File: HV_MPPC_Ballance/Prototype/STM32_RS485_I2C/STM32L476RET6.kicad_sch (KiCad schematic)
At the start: 10 parts, among them SW1 SW_Push, U1 STM32L476RET6

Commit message: .
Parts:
- C1, C2, C3, C4, C5, C6: footprint Capacitor_SMD:C_0402_1005Metric -> 0_lib:0402_density_C_Capacitor
- R1, R2: footprint Resistor_SMD:R_0402_1005Metric -> 0_lib:0402_density_C_Resistor
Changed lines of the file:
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@@
 			)
 		)
-		(property "Footprint" "Resistor_SMD:R_0402_1005Metric"
+		(property "Footprint" "0_lib:0402_density_C_Resistor"
 			(at 37.592 55.88 90)
 			(effects
@@
 			)
 		)
-		(property "Footprint" "Capacitor_SMD:C_0402_1005Metric"
+		(property "Footprint" "0_lib:0402_density_C_Capacitor"
 			(at 70.8152 31.75 0)
 			(effects
@@
 			)
 		)
-		(property "Footprint" "Capacitor_SMD:C_0402_1005Metric"
+		(property "Footprint" "0_lib:0402_density_C_Capacitor"
 			(at 83.5152 31.75 0)
 			(effects
@@
 			)
 		)
-		(property "Footprint" "Capacitor_SMD:C_0402_1005Metric"
+		(property "Footprint" "0_lib:0402_density_C_Capacitor"
 			(at 58.1152 31.75 0)
 			(effects
@@
 			)
 		)
-		(property "Footprint" "Capacitor_SMD:C_0402_1005Metric"
+		(property "Footprint" "0_lib:0402_density_C_Capacitor"
 			(at 89.8652 31.75 0)
 			(effects
@@
 			)
 		)
-		(property "Footprint" "Capacitor_SMD:C_0402_1005Metric"
+		(property "Footprint" "0_lib:0402_density_C_Capacitor"
 			(at 77.1652 31.75 0)
 			(effects
@@
 			)
 		)
-		(property "Footprint" "Capacitor_SMD:C_0402_1005Metric"
+		(property "Footprint" "0_lib:0402_density_C_Capacitor"
 			(at 64.4652 31.75 0)
 			(effects
@@
 			)
 		)
-		(property "Footprint" "Resistor_SMD:R_0402_1005Metric"
+		(property "Footprint" "0_lib:0402_density_C_Resistor"
 			(at 43.942 69.85 90)
 			(effects

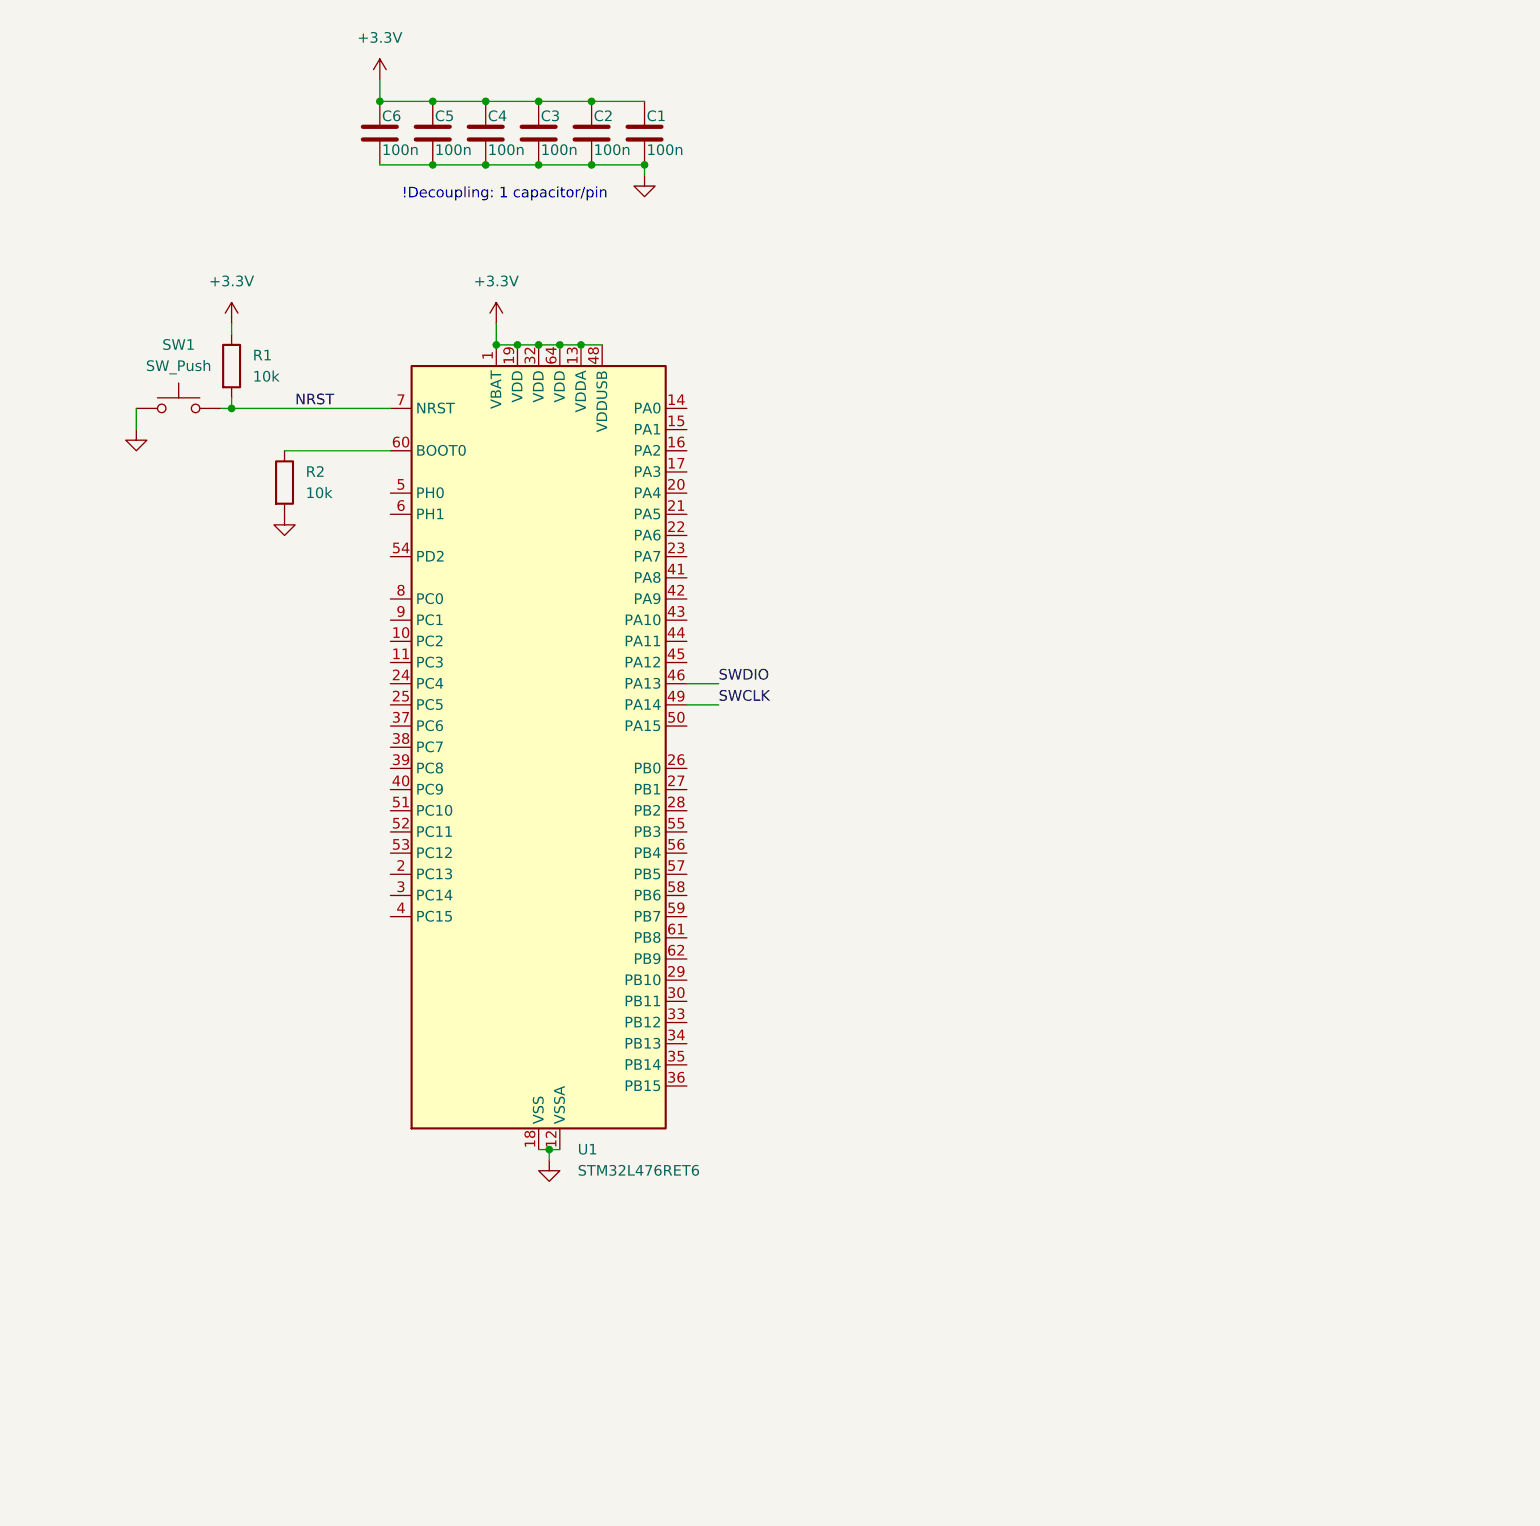
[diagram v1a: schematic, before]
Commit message: .
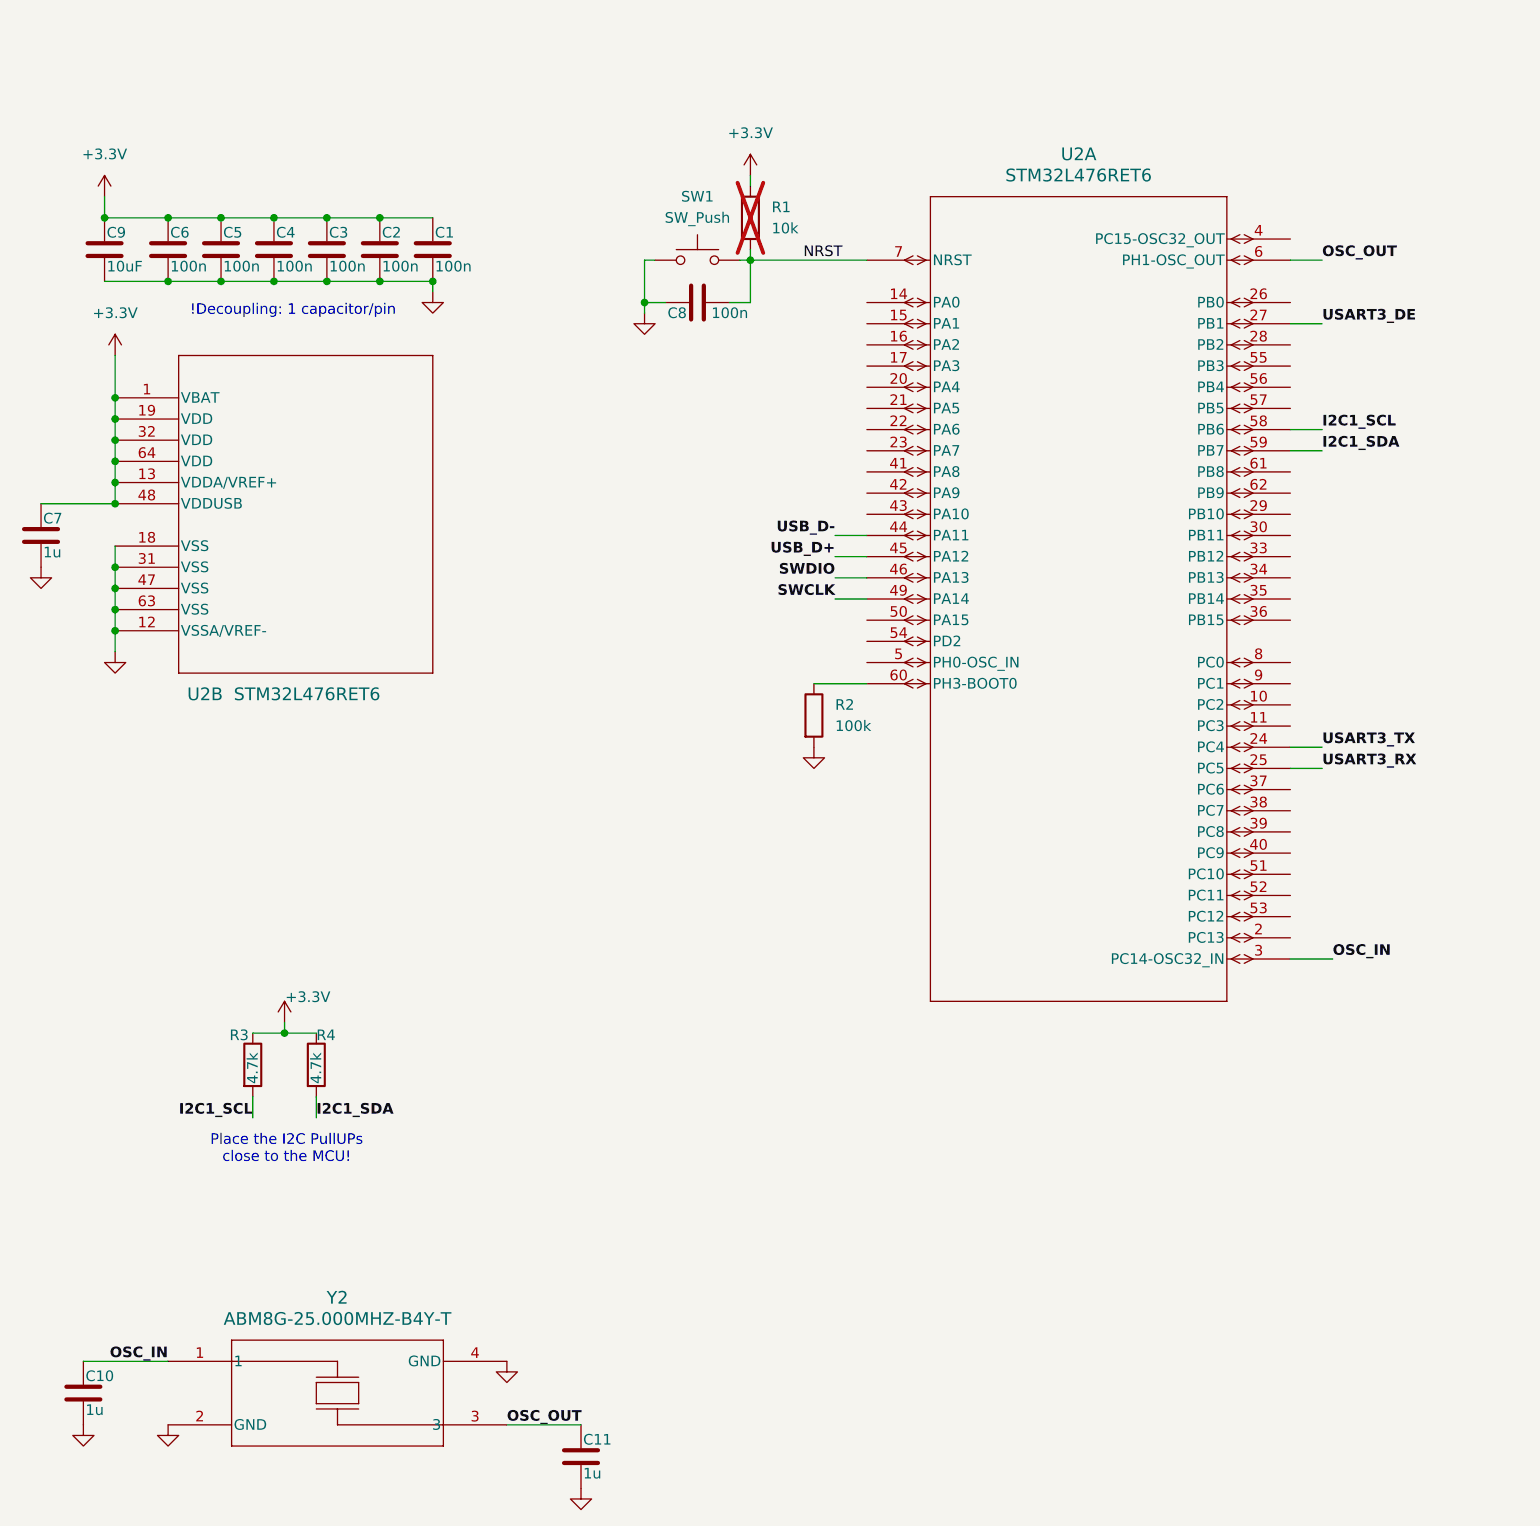
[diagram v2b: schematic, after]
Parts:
- removed U1: STM32L476RET6, Package_QFP:LQFP-64_10x10mm_P0.5mm, symbol MCU_ST_STM32L4:STM32L476RETx
- added C10, C11, C7: 1u, 0_lib:0402_density_C_Capacitor, symbol Device:C
- added C8: 100n, 0_lib:0402_density_C_Capacitor, symbol Device:C
- added C9: 10uF, 0_lib:0402_density_C_Capacitor, symbol Device:C
- added R3, R4: 4.7k, 0_lib:0402_density_C_Resistor, symbol Device:R
- added U2: STM32L476RET6, 0_lib:STM32L476RET6-LQFP64-10x10mm_STM, symbol 0-lib:STM32L476RET6
- added Y2: ABM8G-25.000MHZ-B4Y-T, CRYSTAL_ABM8G_ABR, symbol 0-lib:ABM8G-25.000MHZ-B4Y-T
- R1: now not fitted
- R2: value 10k -> 100k
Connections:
- net +3.3V: now also C7.1, C9.1, R3.1, R4.1, U2.1 (VBAT), U2.13 (VDDA/VREF+), U2.19 (VDD), U2.32 (VDD), U2.48 (VDDUSB), U2.64 (VDD)
- net GND: now also C10.2, C11.2, C7.2, C8.1, C9.2, U2.12 (VSSA/VREF-), U2.18 (VSS), U2.31 (VSS), U2.47 (VSS), U2.63 (VSS), Y2.2 (GND), Y2.4 (GND)
- net NRST: now also C8.2, U2.7 (NRST)
- net SWCLK: now also U2.49 (PA14)
- net SWDIO: now also U2.46 (PA13)
- net at R2.1: now also U2.60 (PH3-BOOT0)
- new net I2C1_SCL: R3.2, U2.58 (PB6)
- new net I2C1_SDA: R4.2, U2.59 (PB7)
- new net OSC_IN: C10.1, U2.3 (PC14-OSC32_IN), Y2.1
- new net OSC_OUT: C11.1, U2.6 (PH1-OSC_OUT), Y2.3
- new net USART3_DE: U2.27 (PB1)
- new net USART3_RX: U2.25 (PC5)
- new net USART3_TX: U2.24 (PC4)
- new net USB_D+: U2.45 (PA12)
- new net USB_D-: U2.44 (PA11)
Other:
- note added: "Place the I2C PullUPs close to the MCU!"
- moved on the sheet: C1, C2, C3, C4, C5, C6, R2, SW1

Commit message: .
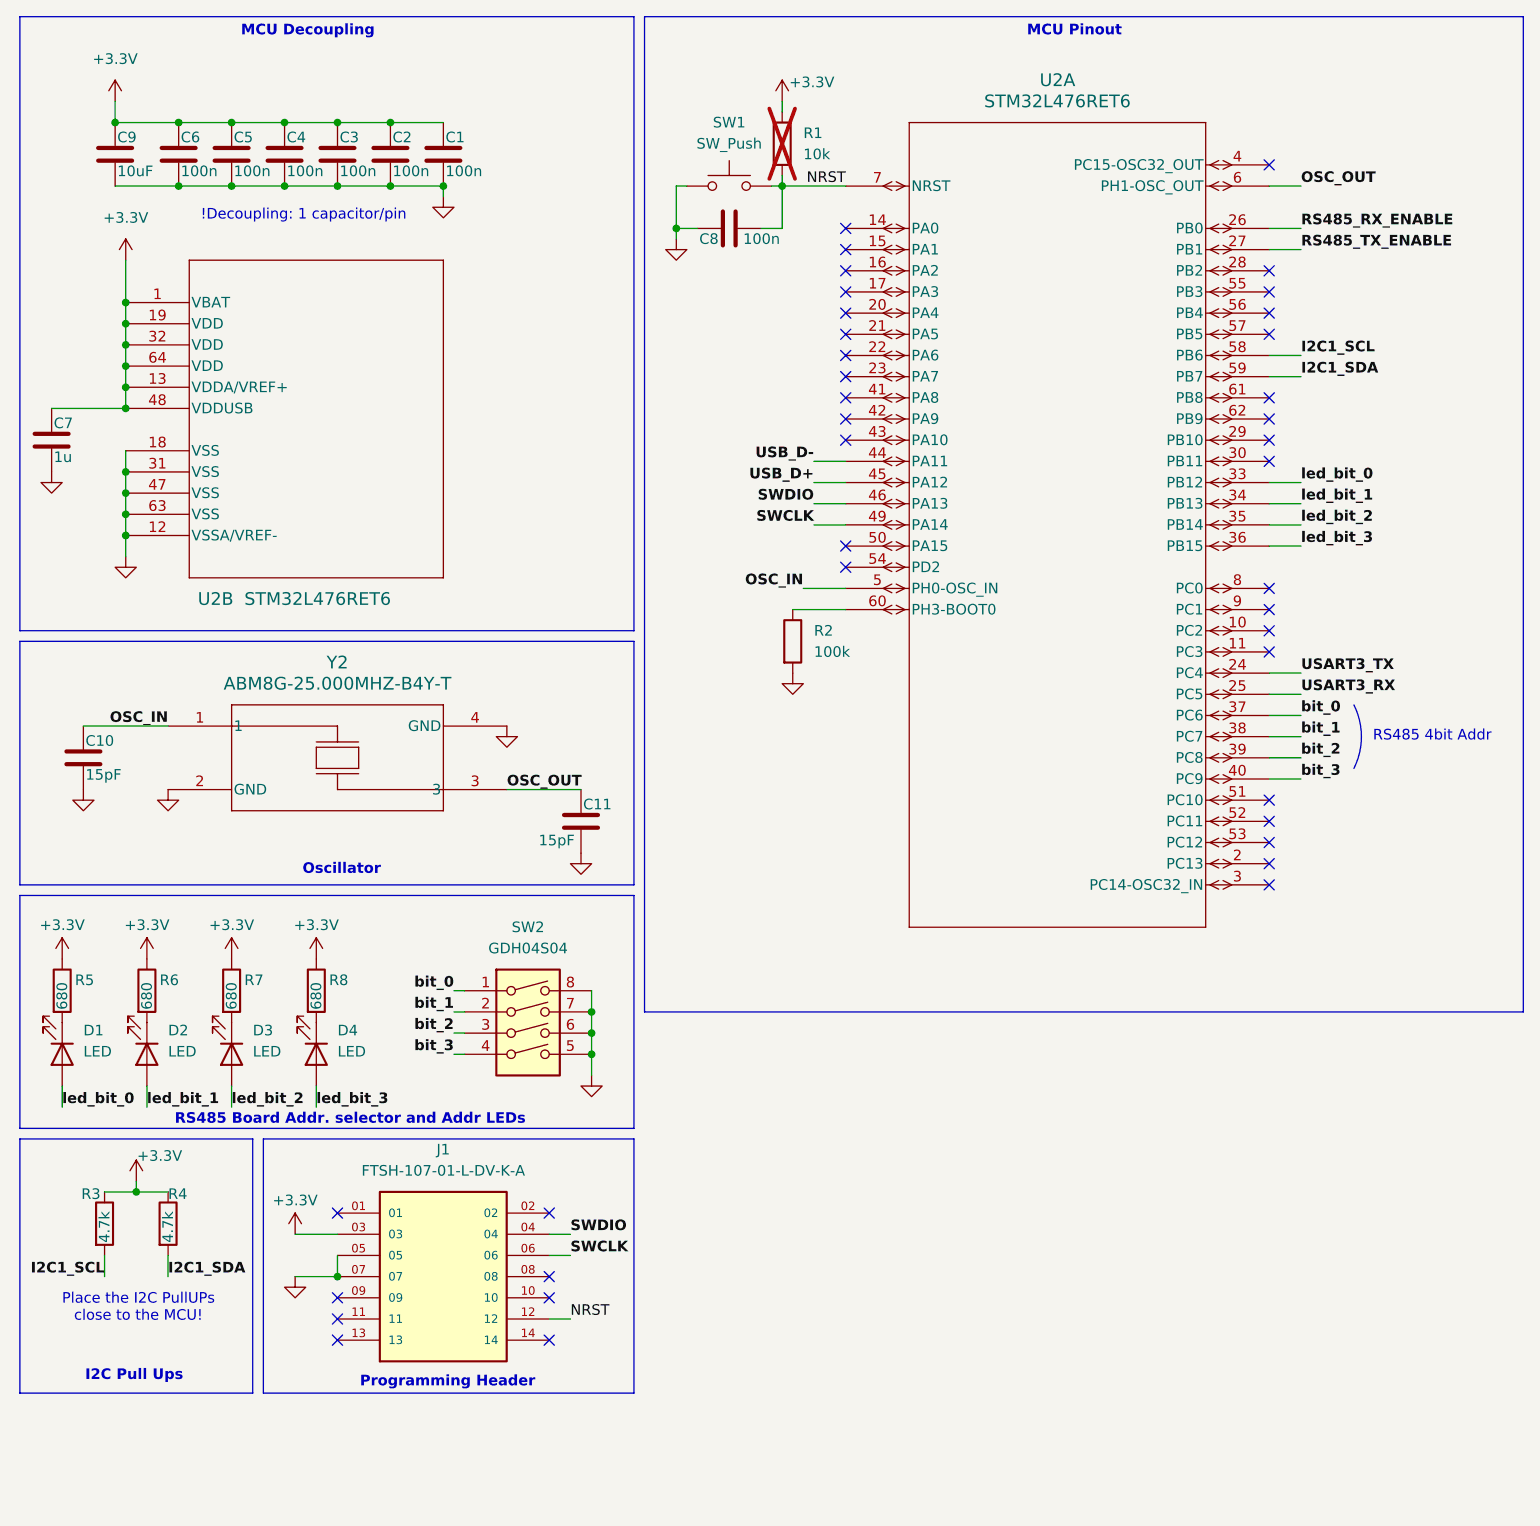
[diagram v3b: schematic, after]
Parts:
- added D1, D2, D3, D4: LED, LED_SMD:LED_0402_1005Metric, symbol Device:LED
- added J1: FTSH-107-01-L-DV-K-A, 0_lib:SAMTEC_FTSH-107-01-L-DV-K-A, symbol 0-lib:FTSH-107-01-L-DV-K-A
- added R5, R6, R7, R8: 680, 0_lib:0402_density_C_Resistor, symbol Device:R
- added SW2: GDH04S04, 0_lib:GDH04S04, symbol Switch:SW_DIP_x04
- C10, C11: value 1u -> 15pF
- Y2: footprint CRYSTAL_ABM8G_ABR -> 0_lib:CRYSTAL_ABM8G_ABR
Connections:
- net +3.3V: now also J1.03, R5.1, R6.1, R7.1, R8.1
- net GND: now also J1.05, J1.07, SW2.5, SW2.6, SW2.7, SW2.8
- net NRST: now also J1.12
- net OSC_IN: now also U2.5 (PH0-OSC_IN); no longer U2.3 (PC14-OSC32_IN)
- net SWCLK: now also J1.06
- net SWDIO: now also J1.04
- net RS485_RX_ENABLE: now reaches U2.26 (PB0)
- net led_bit_0: now reaches U2.33 (PB12)
- net led_bit_0: now also D1.2 (A)
- net led_bit_1: now reaches U2.34 (PB13)
- net led_bit_1: now also D2.2 (A)
- net led_bit_2: now reaches U2.35 (PB14)
- net led_bit_2: now also D3.2 (A)
- net led_bit_3: now reaches U2.36 (PB15)
- net led_bit_3: now also D4.2 (A)
- net bit_0: now reaches U2.37 (PC6)
- net bit_0: now also SW2.1
- net bit_1: now reaches U2.38 (PC7)
- net bit_1: now also SW2.2
- net bit_2: now reaches U2.39 (PC8)
- net bit_2: now also SW2.3
- net bit_3: now reaches U2.40 (PC9)
- net bit_3: now also SW2.4
- net USART3_DE renamed RS485_TX_ENABLE
- new net: D2.1 (K), R6.2
- new net: D1.1 (K), R5.2
- new net: D3.1 (K), R7.2
- new net: D4.1 (K), R8.2
- no-connect marks 0 -> 39
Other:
- note added: "I2C Pull Ups"
- note added: "MCU Decoupling"
- note added: "MCU Pinout"
- note added: "Oscillator"
- note added: "Programming Header"
- note added: "RS485 4bit Addr"
- note added: "RS485 Board Addr. selector and Addr LEDs"
- title: (none) -> Microcontroller
- moved on the sheet: C1, C10, C11, C2, C3, C4, C5, C6, C7, C8, C9, R1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
